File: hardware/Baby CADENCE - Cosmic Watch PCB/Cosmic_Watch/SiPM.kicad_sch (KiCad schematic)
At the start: 1 part, among them IC1 MICROFJ-60035-TSV-TR1

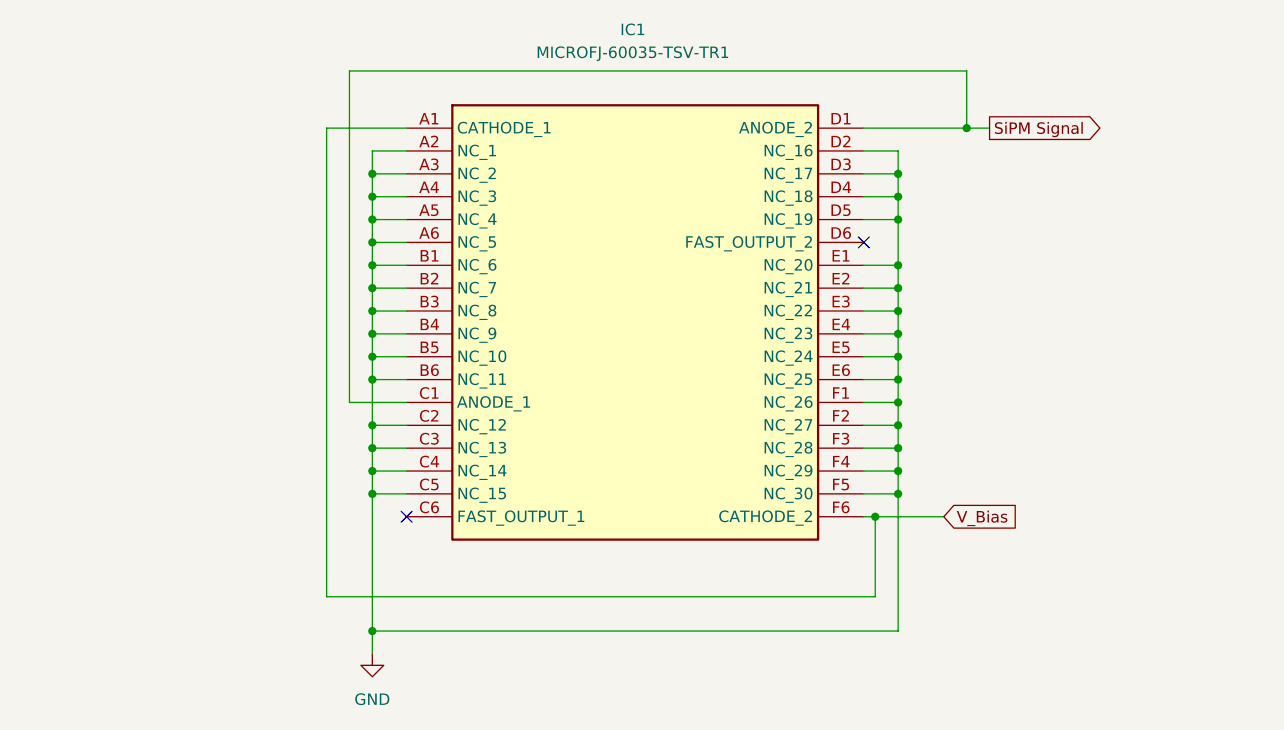
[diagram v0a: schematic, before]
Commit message: Comments/Reminders
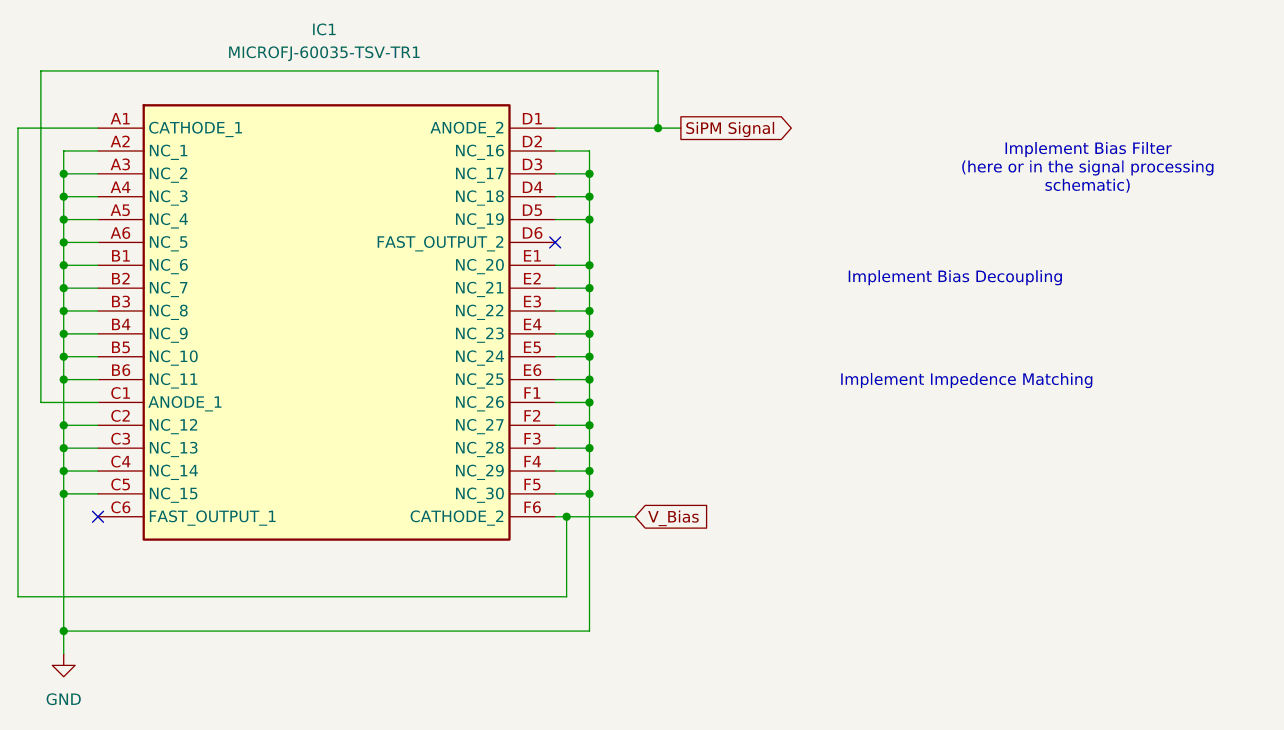
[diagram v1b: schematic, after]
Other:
- note added: "Implement Bias Decoupling"
- note added: "Implement Bias Filter (here or in the signal processing schematic)"
- note added: "Implement Impedence Matching"
- moved on the sheet: IC1
